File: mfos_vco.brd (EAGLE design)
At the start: 100 x 80.8 mm, 60 parts, among them IC1 TL072P, IC2 TL072P, IC3 TL072P, IC4 LM394N, U1 POWER, U2 2N5457

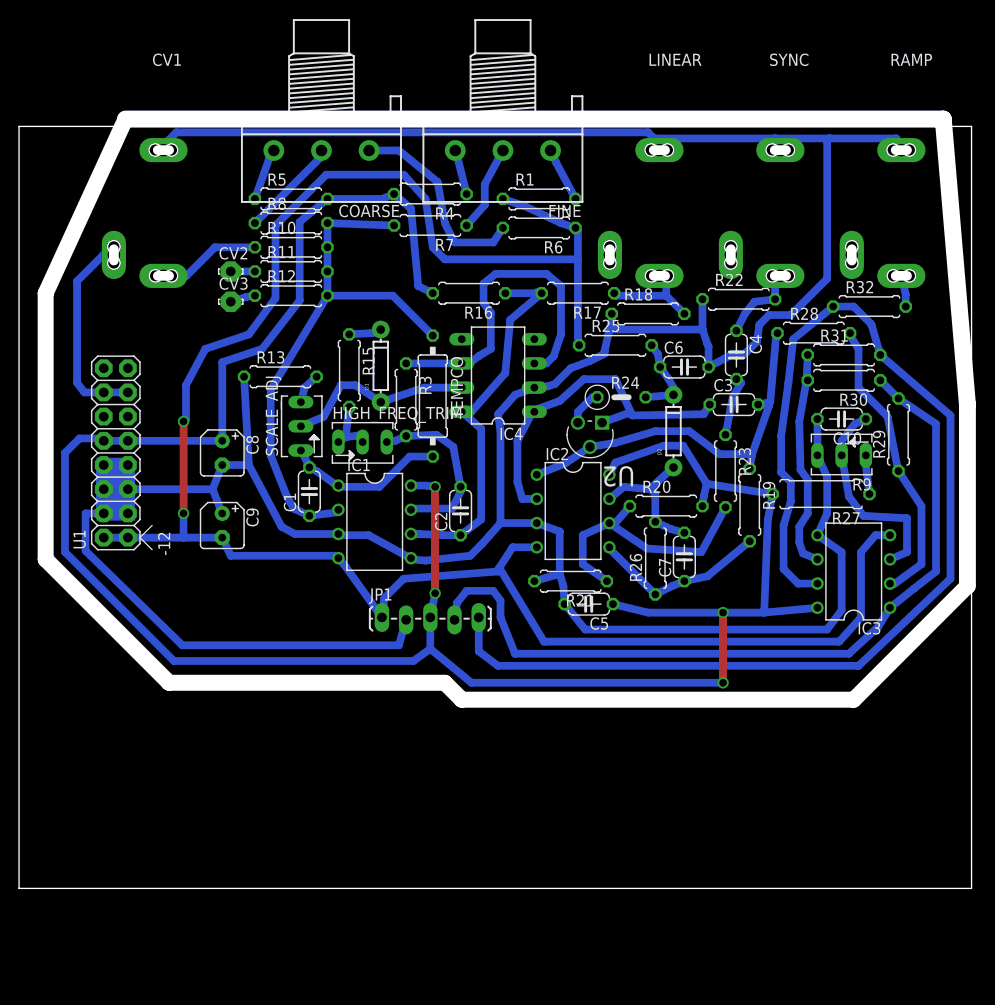
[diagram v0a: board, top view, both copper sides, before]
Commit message: molex
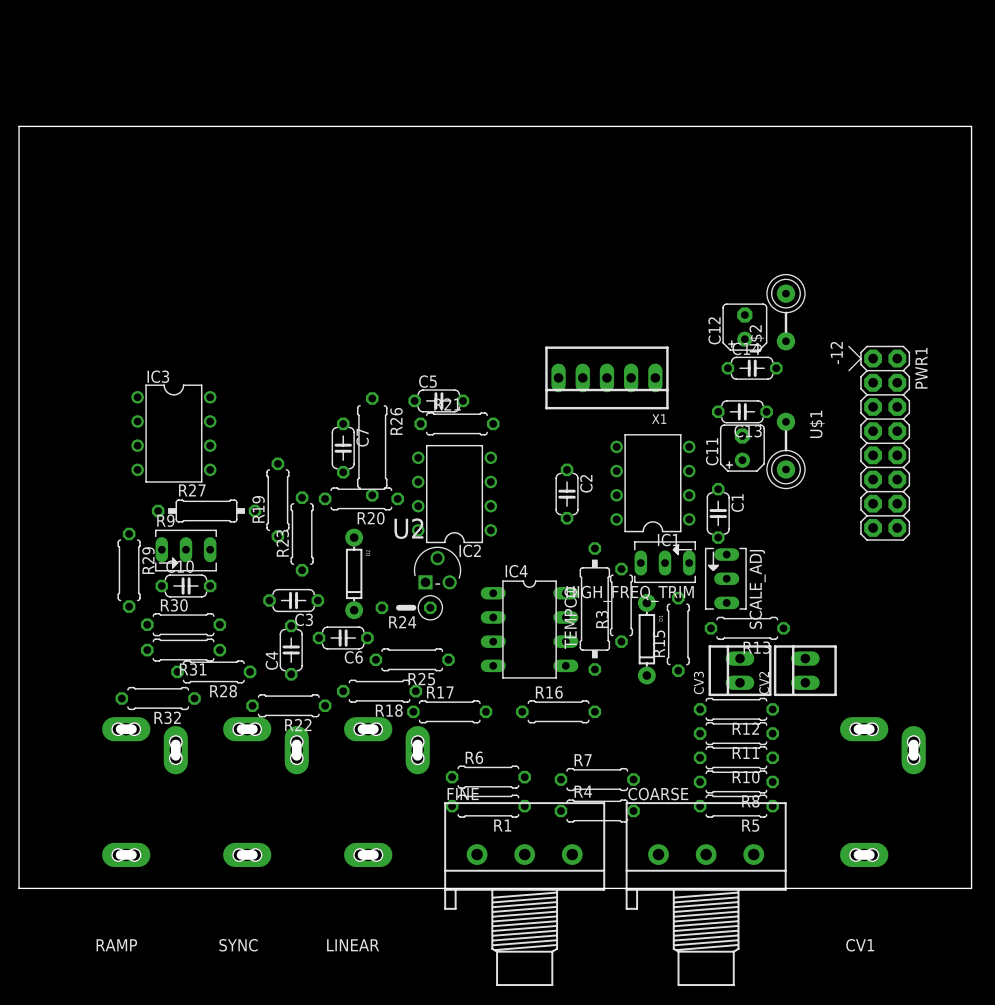
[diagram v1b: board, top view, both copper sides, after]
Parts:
- removed C8, C9: 10uF, rcl:B45181A
- removed JP1: (no value), SparkFun-Connectors:1X05_LOCK_LONGPADS
- removed U1: POWER, eurorack:POWER_16
- added C11, C12: 10u, rcl:B45181A
- added C13, C14: 100n, rcl:C050-024X044
- added PWR1: POWER, eurorack:POWER_16
- added U$1, U$2: FB, adafruit:FB
- added X1: 22-23-2051, con-molex:22-23-2051
- CV2, CV3: value LSP10 -> 22-23-2021; device solpad:LSP10 -> con-molex:22-23-2021
- R26: device rcl:0207/7 -> rcl:0309/10
- R27: device rcl:0309/10 -> rcl:0207/10
- moved CV1 115.0 mm to (93.7, 1.02), turned to 180 degrees
- moved RAMP 106.5 mm to (16.3, 1.02), turned to 180 degrees
- moved SYNC 91.4 mm to (29.0, 1.02), turned to 180 degrees
- moved R32 85.3 mm to (14.6, 19.9), turned to 180 degrees
- moved COARSE 84.2 mm to (72.1, 3.56), turned to 0 degrees
- moved R29 82.0 mm to (11.6, 33.4), turned to 270 degrees
- moved LINEAR 81.6 mm to (41.7, 1.02), turned to 180 degrees
- moved R5 79.0 mm to (75.3, 8.64), turned to 180 degrees
- moved R31 76.0 mm to (17.3, 25.0), turned to 180 degrees
- moved R8 75.0 mm to (75.3, 11.2), turned to 180 degrees
- moved FINE 73.9 mm to (53.1, 3.56), turned to 0 degrees
- moved R30 73.9 mm to (17.3, 27.7), turned to 0 degrees
- moved CV2 73.5 mm to (82.5, 22.9), turned to 90 degrees
- moved IC3 72.8 mm to (16.3, 47.8), turned to 270 degrees
- moved R28 72.3 mm to (20.4, 22.7), turned to 180 degrees
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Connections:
- new net N$38: PWR1.10, PWR1.9, U$1.P$1
- new net N$39: PWR1.1, PWR1.2, U$2.P$1
- net +12V: now also C11.+, C13.1, U$1.P$2, X1.3; no longer C8.+, JP1.3, U1.10, U1.9
- net -12V: now also C12.-, C14.2, U$2.P$2, X1.1; no longer C9.-, JP1.1, U1.1, U1.2
- net GND: now also CV2.2, CV3.2, X1.2; no longer C8.-, C9.+, JP1.2, U1.3, U1.4, U1.5, U1.6, U1.7, U1.8
- net N$11: now also PWR1.13, PWR1.14; no longer U1.13, U1.14
- net N$18: now also CV2.1; no longer CV2.MP
- net N$19: now also CV3.1; no longer CV3.MP
- net N$26: now also C11.-, C12.+, C13.2, C14.1, PWR1.3, PWR1.4, PWR1.5, PWR1.6, PWR1.7, PWR1.8
- net N$33: now also X1.4; no longer JP1.4
- net N$35: now also X1.5; no longer JP1.5
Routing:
- net GND: track 350.7 -> 0.00 mm
- net +12V: track 237.6 -> 0.00 mm, vias 4 -> 0
- net -12V: track 206.4 -> 0.00 mm, vias 2 -> 0
- net N$35: track 126.6 -> 0.00 mm
- net N$33: track 84.2 -> 0.00 mm
- net N$10: track 57.4 -> 0.00 mm
- net N$21: track 41.8 -> 0.00 mm
- net N$40: track 40.8 -> 0.00 mm
- net N$23: track 37.5 -> 0.00 mm
- net N$12: track 36.3 -> 0.00 mm
- net N$31: track 31.3 -> 0.00 mm
- net N$26: track 28.0 -> 0.00 mm
- net N$34: track 23.3 -> 0.00 mm
- net N$28: track 22.0 -> 0.00 mm
- net N$11: track 21.5 -> 0.00 mm
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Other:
- board size 100 x 80.8 mm -> 100 x 80 mm
